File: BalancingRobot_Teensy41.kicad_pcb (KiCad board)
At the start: 2 copper layers, 23 parts, among them J1 Conn_01x06_Socket, J2 Conn_01x04_Socket, J3 Conn_01x02_Socket, J4 Conn_01x06_Socket, J5 Conn_01x06_Socket, U1 Teensy4.1, U3 DRV8874_Carrier, U4 DRV8874_Carrier, U5 ICM20948_Carrier_Board

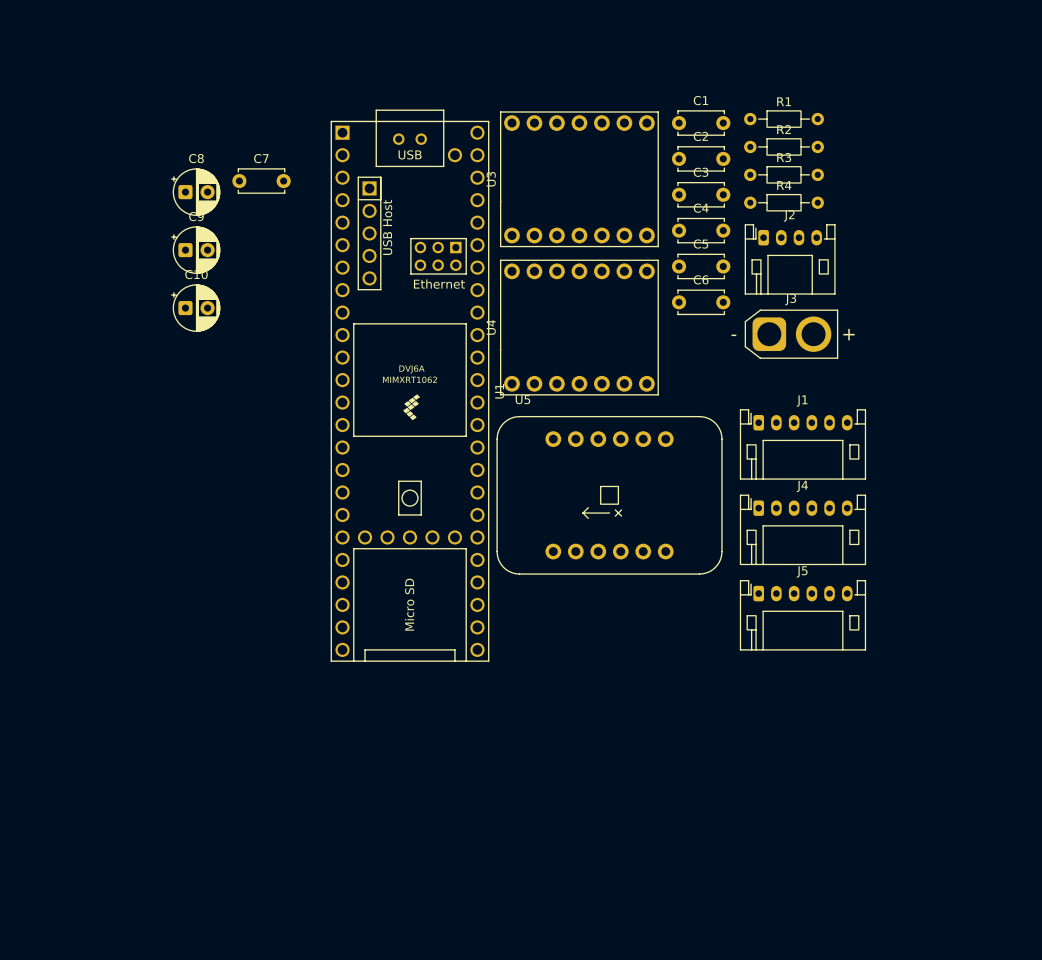
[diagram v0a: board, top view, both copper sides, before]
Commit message: Started with routing
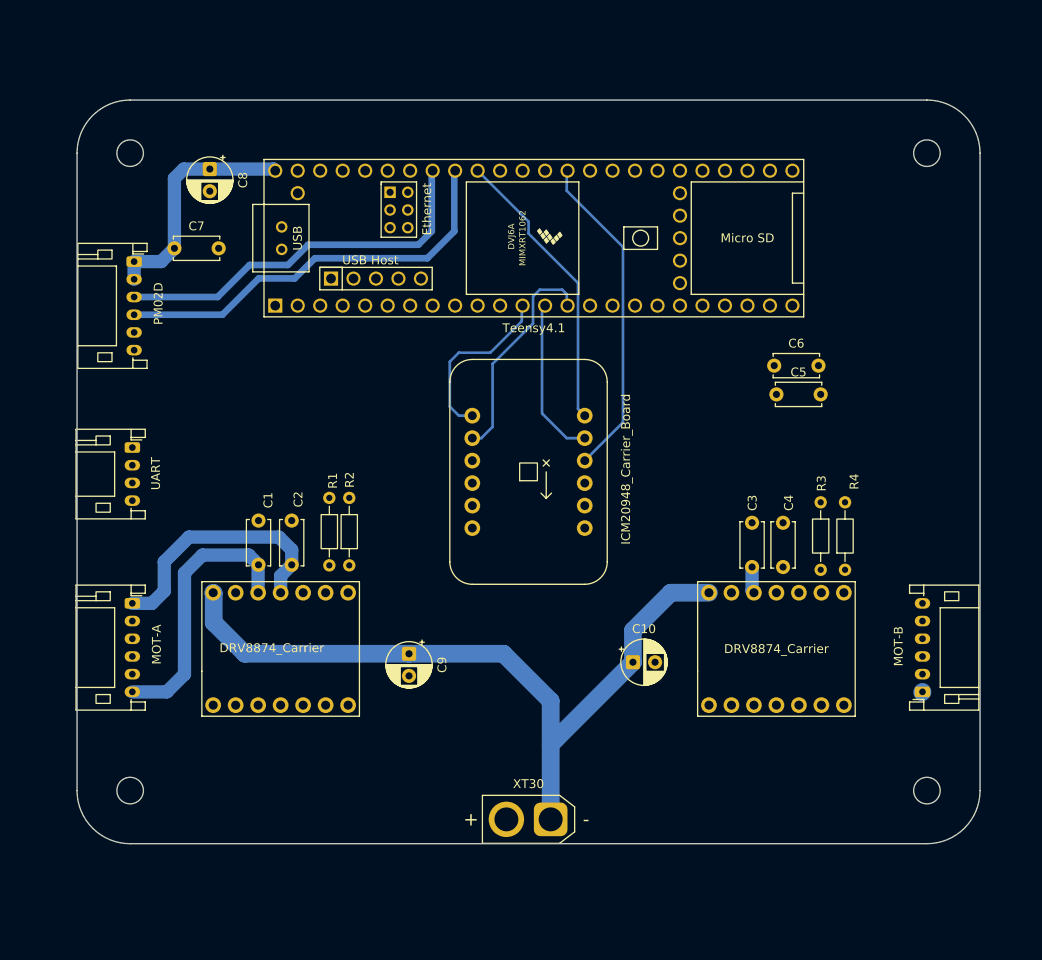
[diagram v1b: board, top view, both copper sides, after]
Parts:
- J1: value Conn_01x06_Socket -> PM02D
- J2: value Conn_01x04_Socket -> UART
- J3: value Conn_01x02_Socket -> XT30
- J4: value Conn_01x06_Socket -> MOT-A
- J5: value Conn_01x06_Socket -> MOT-B
- moved J2 75.1 mm to (105.2, 97.2), turned to -90 degrees
- moved J1 72.9 mm to (105.5, 76.2), turned to -90 degrees
- moved J4 71.6 mm to (105.2, 114.8), turned to -90 degrees
- moved C1 68.9 mm to (119.5, 110.5), turned to 90 degrees
- moved R2 65.5 mm to (129.8, 110.6), turned to 90 degrees
- moved C10 64.5 mm to (161.8, 121.5)
- moved R1 64.0 mm to (127.5, 102.9), turned to -90 degrees
- moved C2 63.4 mm to (123.2, 110.5), turned to 90 degrees
- moved U3 62.9 mm to (122.0, 120.0)
- moved J3 60.1 mm to (152.5, 139.2), turned to 180 degrees
- moved C9 52.1 mm to (136.5, 120.5), turned to -90 degrees
- moved C3 42.9 mm to (175.2, 110.8), turned to 90 degrees
- moved R4 42.8 mm to (185.8, 111.1), turned to 90 degrees
- moved U4 42.6 mm to (178.0, 120.0)
- moved C4 39.8 mm to (178.8, 110.8), turned to 90 degrees
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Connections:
- U1 pad 66: unconnected-(U1-D--Pad66) -> (no net)
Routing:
- net +12V: track 0.00 -> 85.6 mm
- net PM02_SDA: track 0.00 -> 47.0 mm
- net PM02_SCL: track 0.00 -> 43.6 mm
- net ICM20948_SCL: track 0.00 -> 37.2 mm
- net ICM20948_INT: track 0.00 -> 32.7 mm
- net Net-(J4-M-): track 0.00 -> 31.0 mm
- net Net-(J4-M+): track 0.00 -> 29.0 mm
- net +5V: track 0.00 -> 27.0 mm
- net ICM20948_SDO: track 0.00 -> 25.1 mm
- net ICM20948_CS: track 0.00 -> 19.9 mm
- net ICM20948_SDI: track 0.00 -> 18.7 mm
- net Net-(J5-M-): track 0.00 -> 2.99 mm
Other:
- board outline added: 102 x 84 mm

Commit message: Almost completed with routing
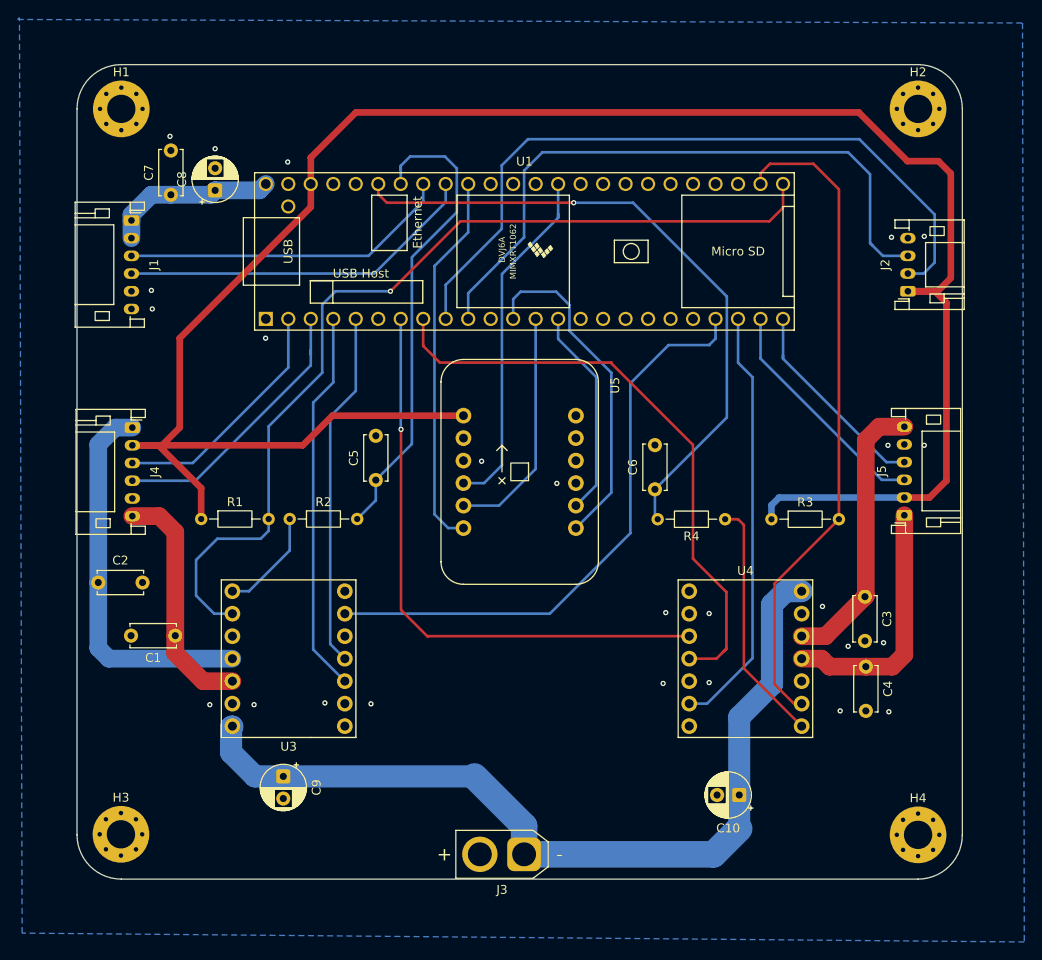
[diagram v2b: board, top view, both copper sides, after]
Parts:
- added H1: MountingHole_Pad, MountingHole:MountingHole_3.2mm_M3_Pad_Via, F.Cu at (104.0, 59.0)
- added H2: MountingHole_Pad, MountingHole:MountingHole_3.2mm_M3_Pad_Via, F.Cu at (194.0, 59.0)
- added H3: MountingHole_Pad, MountingHole:MountingHole_3.2mm_M3_Pad_Via, F.Cu at (104.0, 140.9)
- added H4: MountingHole_Pad, MountingHole:MountingHole_3.2mm_M3_Pad_Via, F.Cu at (194.0, 141.0)
- moved J2 89.4 mm to (192.8, 79.6), turned to 90 degrees
- moved C5 46.3 mm to (132.8, 100.9), turned to 90 degrees
- moved C2 21.9 mm to (101.4, 112.5), turned to 0 degrees
- moved J5 20.1 mm to (192.4, 104.9)
- moved J4 19.8 mm to (105.2, 95.0)
- moved C9 19.8 mm to (122.3, 134.4)
- moved C6 19.4 mm to (164.3, 102.0), turned to 90 degrees
- moved C10 19.2 mm to (173.8, 136.5), turned to 180 degrees
- moved R4 14.7 mm to (172.2, 105.3), turned to 180 degrees
- moved R1 14.7 mm to (113.0, 105.3), turned to 0 degrees
- moved C4 14.6 mm to (188.1, 122.0), turned to -90 degrees
- moved C3 13.2 mm to (188.0, 114.1), turned to -90 degrees
- moved C1 12.3 mm to (110.1, 118.5), turned to 180 degrees
- moved R2 8.52 mm to (123.0, 105.3), turned to 0 degrees
- moved C7 6.06 mm to (109.6, 68.7), turned to 90 degrees
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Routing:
- net +3V3: track 0.00 -> 236.9 mm
- net MOTA_FAULT: track 0.00 -> 105.8 mm, vias 0 -> 1
- net UART_COMP_RX: track 0.00 -> 82.6 mm
- net MOTB_FAULT: track 0.00 -> 74.6 mm
- net MOTB_CUR: track 0.00 -> 74.0 mm, vias 0 -> 1
- net UART_COMP_TX: track 0.00 -> 73.3 mm
- net MOTB_DIR: track 0.00 -> 67.9 mm
- net MOTA_SLEEP: track 0.00 -> 66.9 mm
- net MOTB_PWM: track 0.00 -> 66.7 mm, vias 0 -> 1
- net MOTA_CUR: track 0.00 -> 53.9 mm
- net MOTB_SLEEP: track 0.00 -> 48.3 mm
- net MOTA_PWM: track 0.00 -> 43.3 mm
- net MOTA_DIR: track 0.00 -> 40.3 mm
- net ENC_A_PH_B: track 0.00 -> 31.3 mm
- net Net-(J5-M-): track 2.99 -> 31.7 mm
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- added copper zone on B.Cu, net GND
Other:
- board size 102 x 84 mm -> 100 x 92 mm
